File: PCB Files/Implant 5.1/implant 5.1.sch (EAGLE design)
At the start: 6 parts

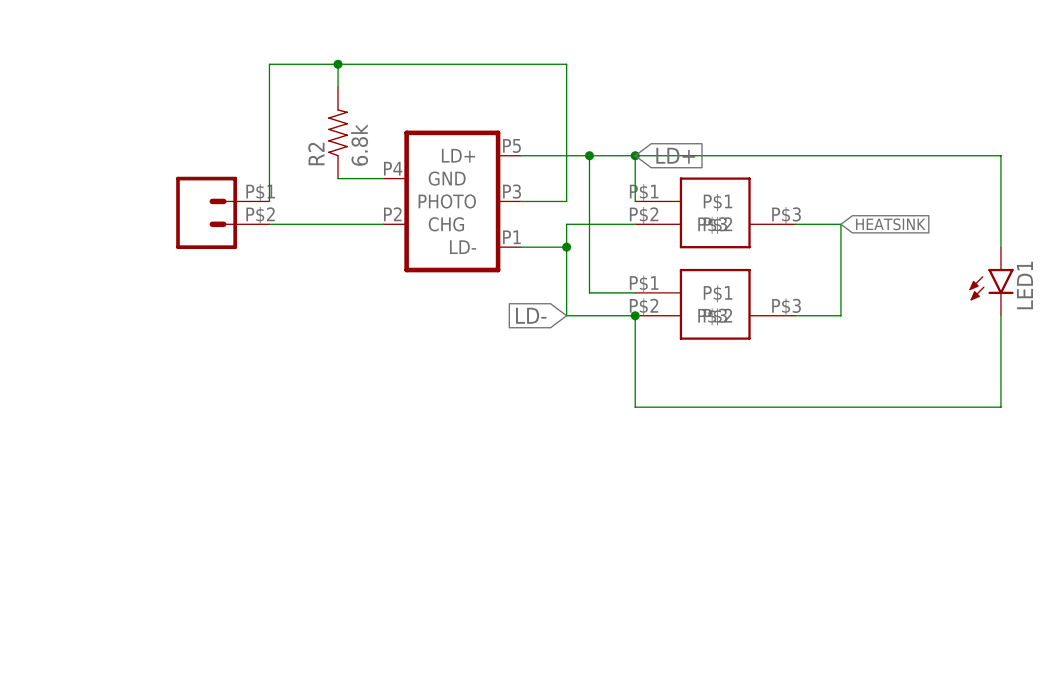
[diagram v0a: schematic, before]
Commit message: update PCB files
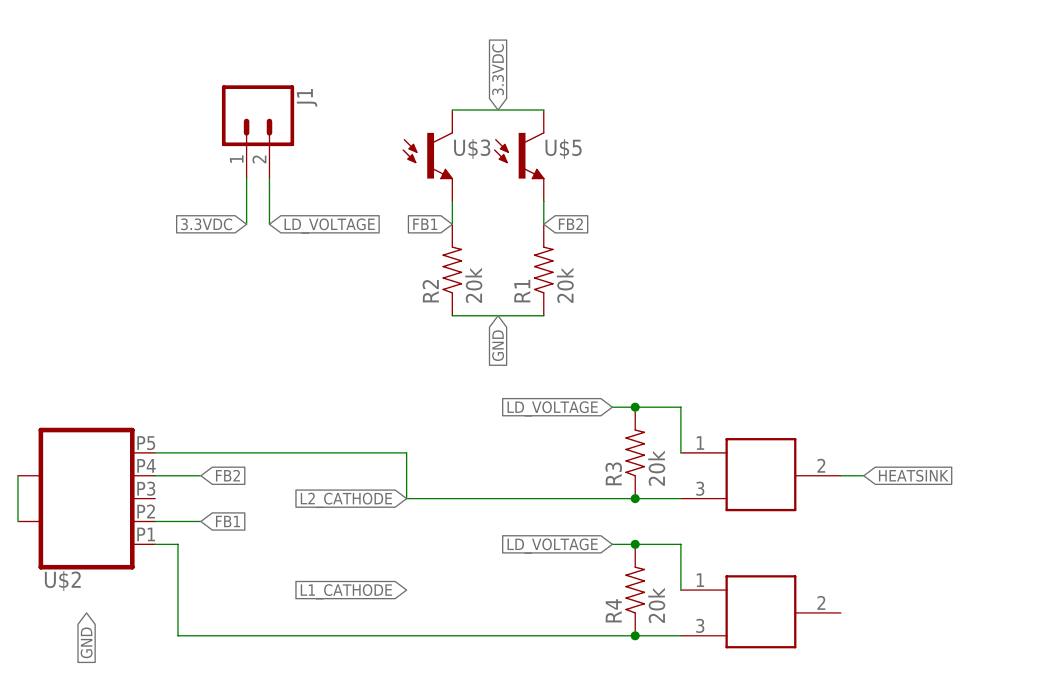
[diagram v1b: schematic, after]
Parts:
- removed JP1: M02SMALL, SparkFun-Connectors:M02SMALL
- removed LED1: (no value), Andy-library:LED10MM
- added J1: (no value), SparkFun-Connectors:CONN_02
- added R1, R3, R4: 20k, Andy-library:RESISTOR0805-RES
- added U$4: LASERDIODE3.8MM, Cerebro-library:LASERDIODE3.8MM
- added U$5: AMBIENT-LIGHT-SENSOR, Cerebro-library:AMBIENT-LIGHT-SENSOR
- R2: value 6.8k -> 20k
- U$1: value LASERDIODE -> LASERDIODE3.8MM; device Andy-library:LASERDIODE -> Cerebro-library:LASERDIODE3.8MM
- U$2: value USB_SOCKET_MICRO_VERT -> USB_MICRO_SOCKET_VERT; device Andy-library:USB_SOCKET_MICRO_VERT -> Cerebro-library:USB_MICRO_SOCKET_VERT
- U$3: value LASERDIODE -> AMBIENT-LIGHT-SENSOR; device Andy-library:LASERDIODE -> Cerebro-library:AMBIENT-LIGHT-SENSOR
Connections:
- removed net LD+: LED1.A, U$1.P$1, U$2.LD+, U$3.P$1
- removed net LD-: LED1.C, U$1.P$2, U$2.LD-, U$3.P$2
- removed net N$1: R2.1, U$2.GND
- removed net N$3: JP1.2, U$2.CHG
- removed net N$4: JP1.1, R2.2, U$2.PHOTO
- new net 3.3VDC: J1.1, U$3.C, U$5.C
- new net FB1: R2.2, U$2.P2, U$3.E
- new net FB2: R1.2, U$2.P4, U$5.E
- new net GND: R1.1, R2.1, U$2.P$1, U$2.P$2
- new net L1_CATHODE: R4.1, U$1.3, U$2.P1
- new net L2_CATHODE: R3.1, U$2.P5, U$4.3
- new net LD_VOLTAGE: J1.2, R3.2, R4.2, U$1.1, U$4.1
- net HEATSINK: now also U$4.2; no longer U$1.P$3, U$3.P$3
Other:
- moved on the sheet: R2
